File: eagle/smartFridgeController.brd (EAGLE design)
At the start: 39.7 x 24.8 mm, 8 parts

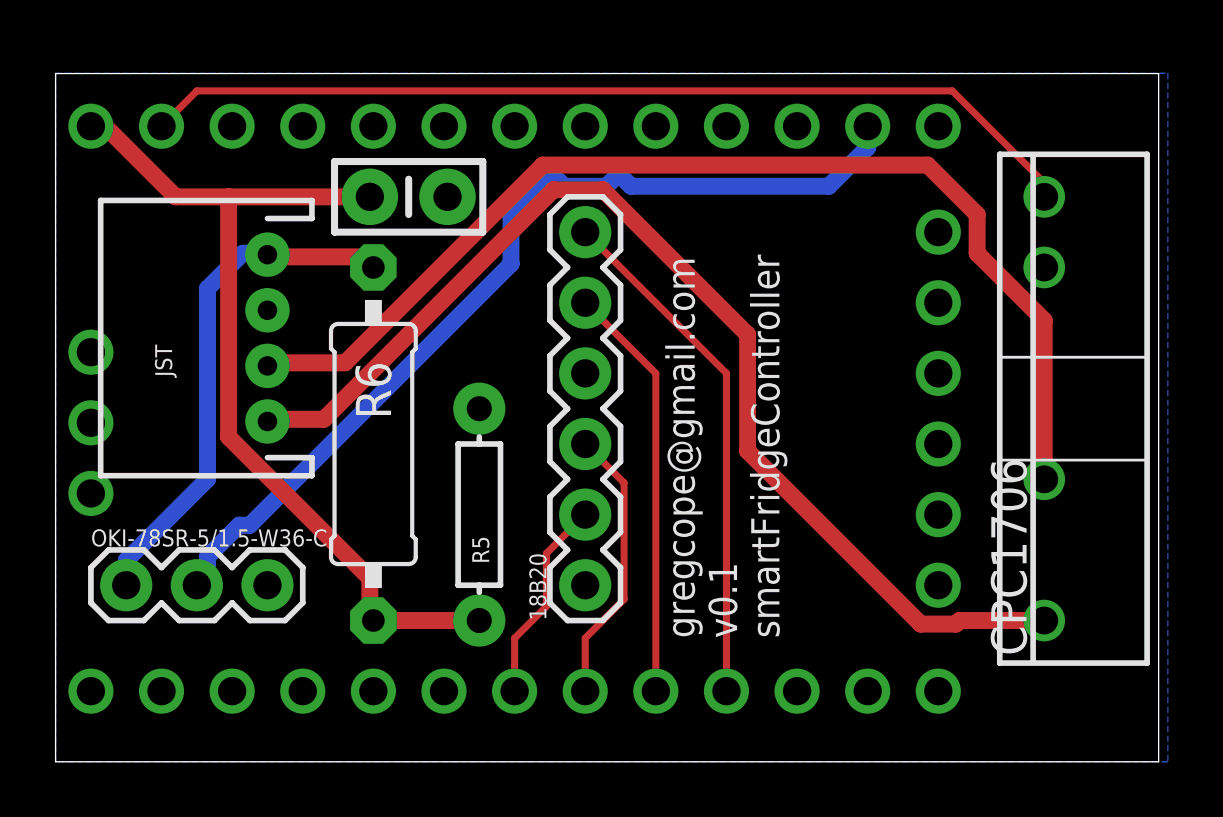
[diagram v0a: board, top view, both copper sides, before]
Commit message: extended board
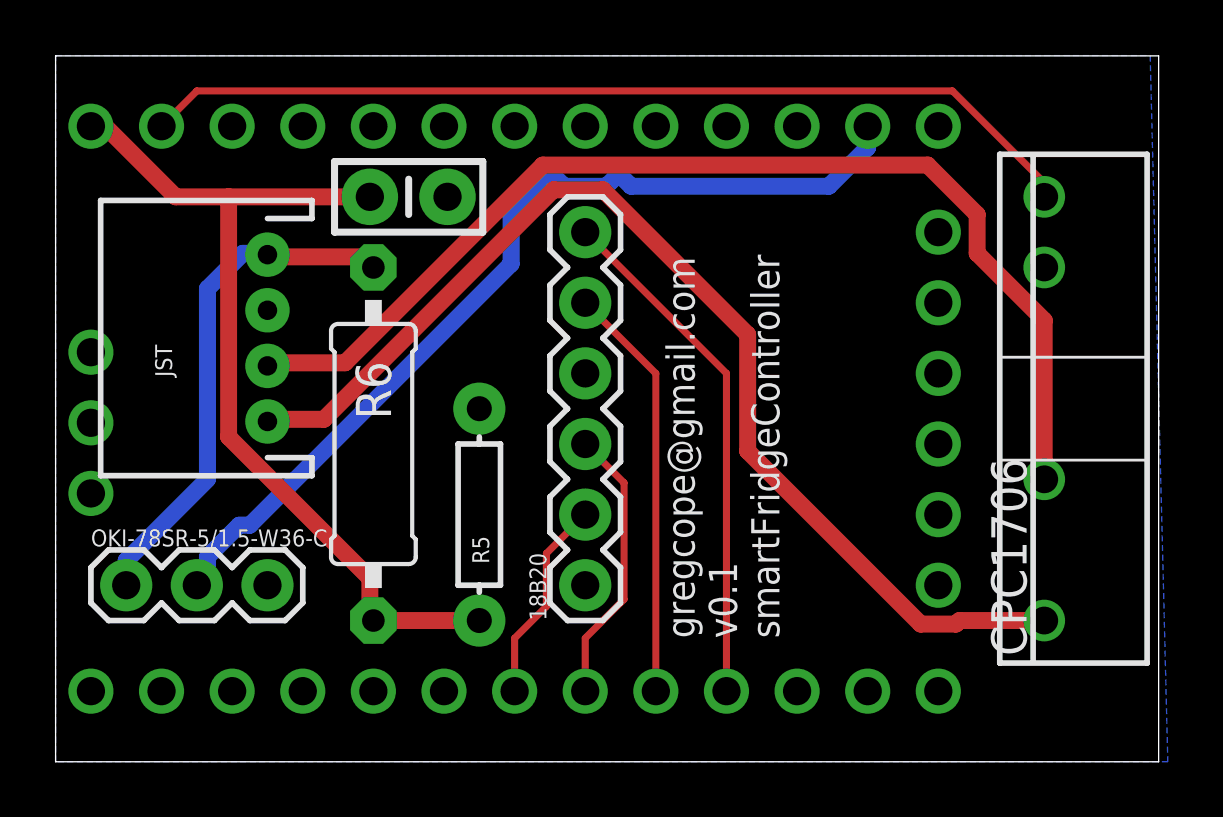
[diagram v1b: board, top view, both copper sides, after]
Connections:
- removed net N$11: U$1.A2
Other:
- board size 39.7 x 24.8 mm -> 39.7 x 25.4 mm
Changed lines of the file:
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@@
 <setting verticaltext="up"/>
 </settings>
-<grid distance="0.05" unitdist="inch" unit="inch" style="lines" multiple="1" display="no" altdistance="0.025" altunitdist="inch" altunit="inch"/>
+<grid distance="0.05" unitdist="inch" unit="inch" style="dots" multiple="1" display="yes" altdistance="0.025" altunitdist="inch" altunit="inch"/>
 <layers>
 <layer number="1" name="Top" color="4" fill="1" visible="yes" active="yes"/>
@@
 <plain>
 <wire x1="0" y1="0" x2="39.675" y2="0" width="0" layer="20"/>
-<wire x1="39.675" y1="0" x2="39.675" y2="24.755" width="0" layer="20"/>
-<wire x1="39.675" y1="24.755" x2="0" y2="24.755" width="0" layer="20"/>
-<wire x1="0" y1="24.755" x2="0" y2="0" width="0" layer="20"/>
+<wire x1="39.675" y1="0" x2="39.675" y2="25.39" width="0" layer="20"/>
+<wire x1="39.675" y1="25.39" x2="0" y2="25.39" width="0" layer="20"/>
+<wire x1="0" y1="25.39" x2="0" y2="0" width="0" layer="20"/>
 <text x="26.035" y="4.445" size="1.016" layer="25" font="vector" rot="R90">gregcope@gmail.com
 v0.1
@@
 <signal name="GND" class="1">
 <polygon width="0.4064" layer="16" isolate="0.3048">
-<vertex x="0" y="24.765"/>
-<vertex x="40.005" y="24.765"/>
+<vertex x="0" y="25.4"/>
+<vertex x="39.37" y="25.4"/>
 <vertex x="40.005" y="0"/>
 <vertex x="0" y="0"/>
@@
 <wire x1="3.81" y1="22.86" x2="5.08" y2="24.13" width="0.254" layer="1"/>
 </signal>
-<signal name="N$11">
-<contactref element="U$1" pad="A2"/>
-</signal>
 <signal name="D5_DS2_PWR">
 <contactref element="U$1" pad="D5"/>
@@
 </signal>
 </signals>
+<errors>
+</errors>
 </board>
 </drawing>
